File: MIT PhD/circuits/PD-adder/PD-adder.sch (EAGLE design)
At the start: 51 parts, among them U1 INA105KP, U2 OP27EZ, U3 OP27EZ, U4 OP27EZ, U5 INA105KP, U6 OP27EZ, U7 REF01EZ, U8 OP27EZ

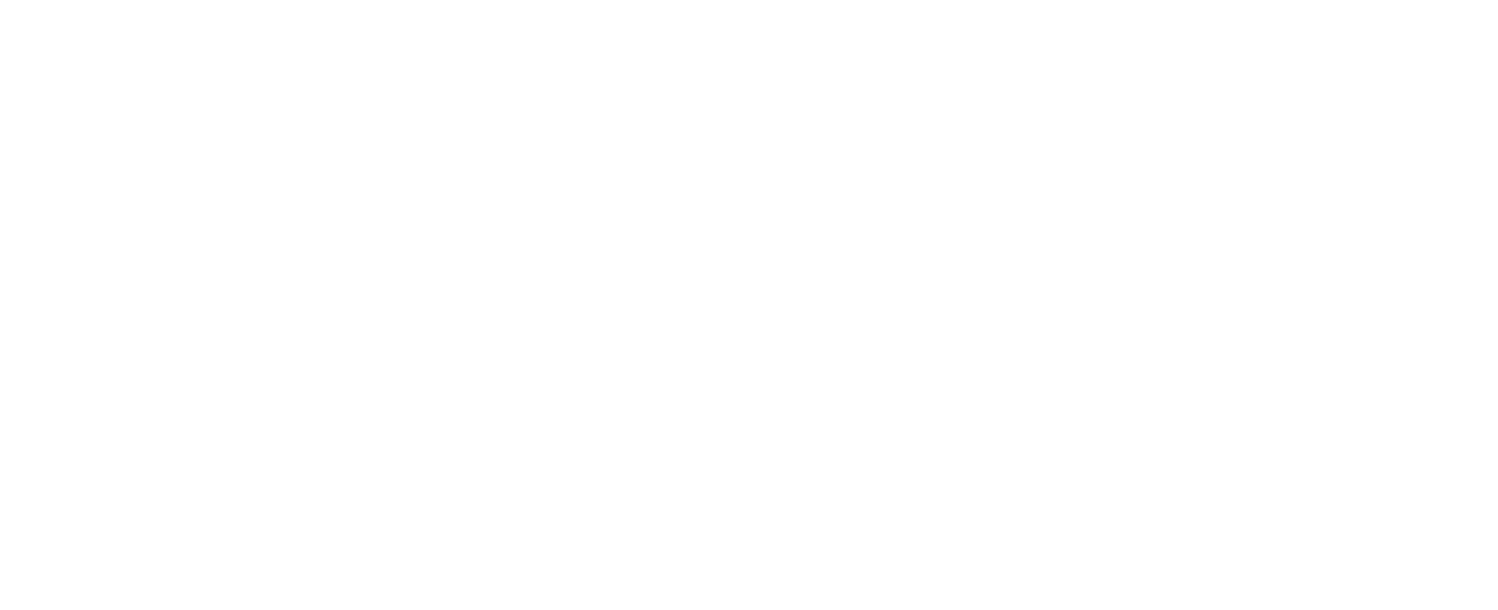
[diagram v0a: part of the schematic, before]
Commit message: circuits
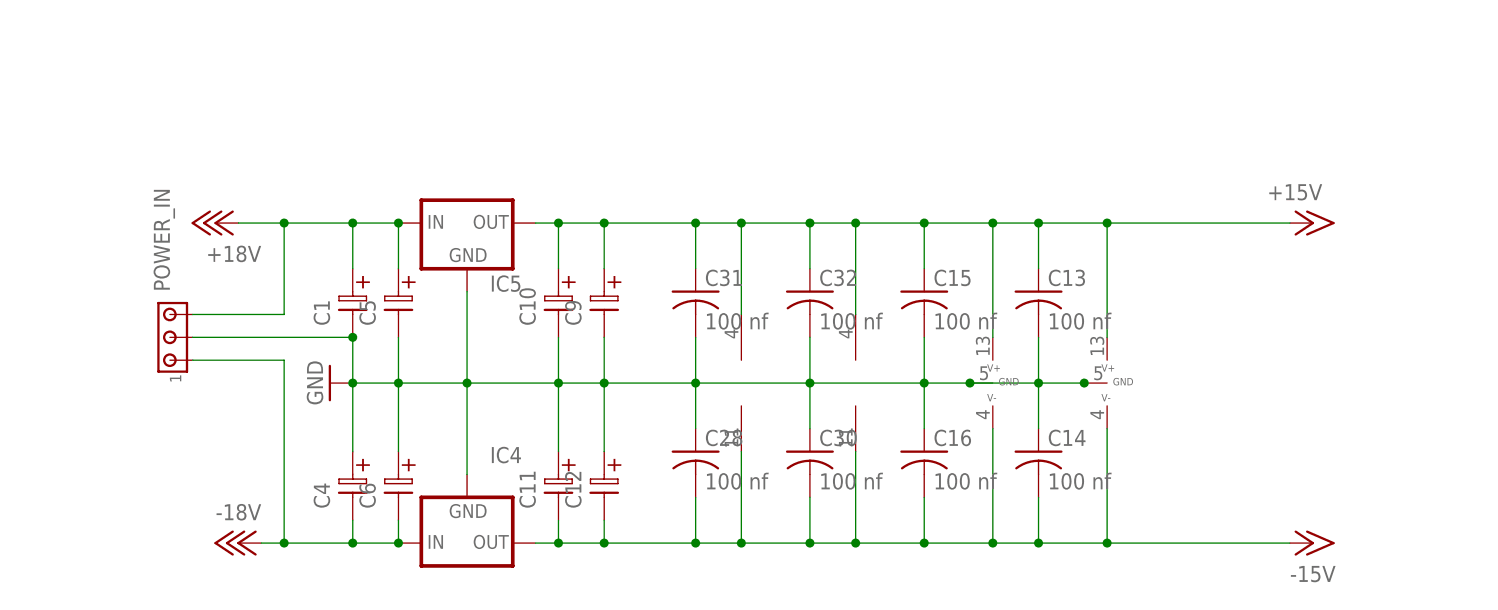
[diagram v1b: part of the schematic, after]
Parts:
- added C1, C10, C11, C12, C4, C5, C6, C9: (no value), discrete:ELC-2,5
- added C13, C14, C15, C16, C28, C30, C31, C32: 100 nf, rcl:C-USC0805
- added IC1: ADG221KN, linear:ADG221KN
- added IC4: (no value), v-reg:79XXL
- added IC5: (no value), v-reg:78XXL
- added IC6, IC7: LF347N, linear:LF347N
- added IC8: ADG222KN, linear:ADG222KN
- added POWER_IN: (no value), con-amp:MTA03-100
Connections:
- new net +18V: C1.1, C5.1, IC5.IN, POWER_IN.3
- new net -18V: C4.2, C6.2, IC4.IN, POWER_IN.1
- net +15V: now also C10.1, C13.1, C15.1, C31.1, C32.1, C9.1, IC1P.V+, IC5.OUT, IC6P.V+, IC7P.V+, IC8P.V+
- net -15V: now also C11.2, C12.2, C14.2, C16.2, C28.2, C30.2, IC1P.V-, IC4.OUT, IC6P.V-, IC7P.V-, IC8P.V-
- net GND: now also C1.2, C10.2, C11.1, C12.1, C13.2, C14.1, C15.2, C16.1, C28.1, C30.1, C31.2, C32.2, C4.1, C5.2, C6.1, C9.2, IC1P.GND, IC4.GND, IC5.GND, IC8P.GND, POWER_IN.2

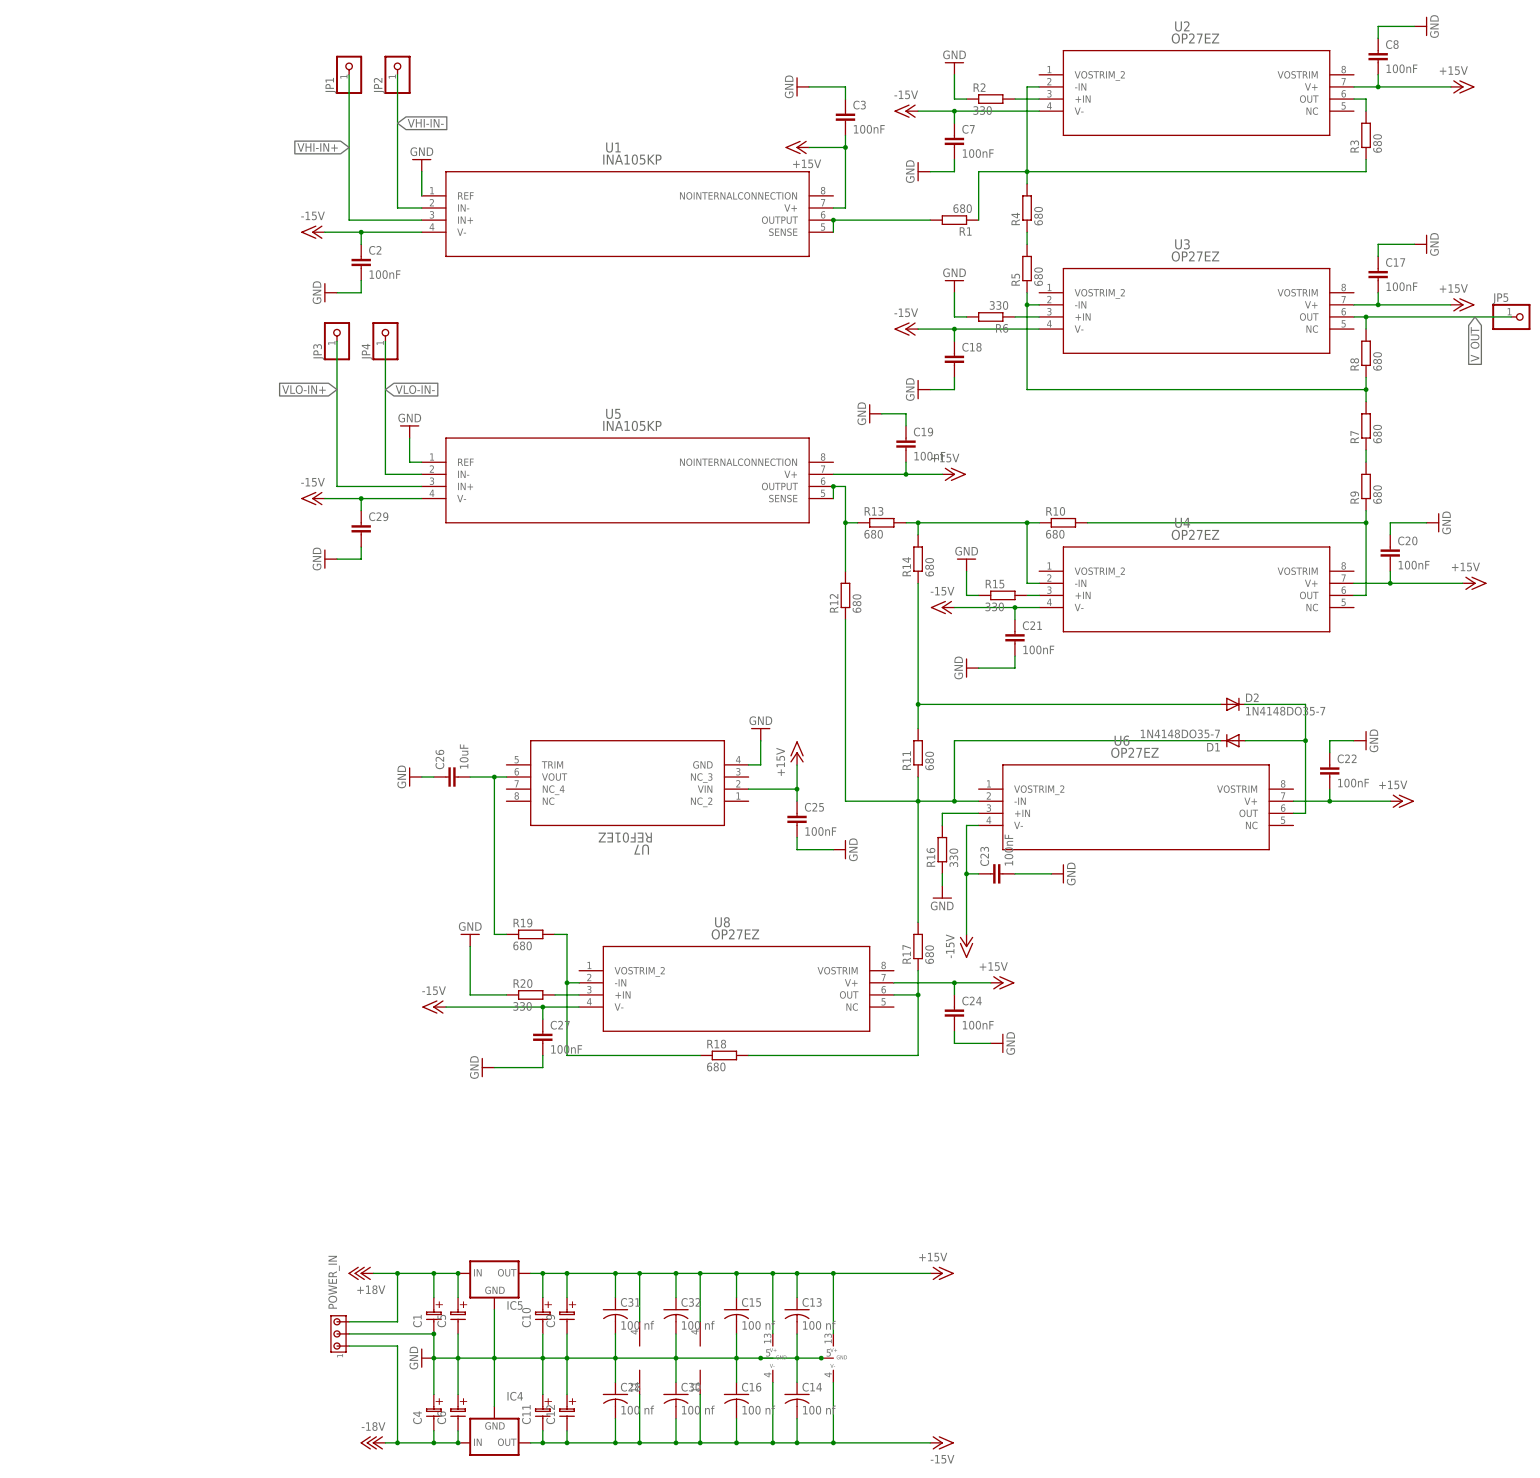
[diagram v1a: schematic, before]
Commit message: circuits
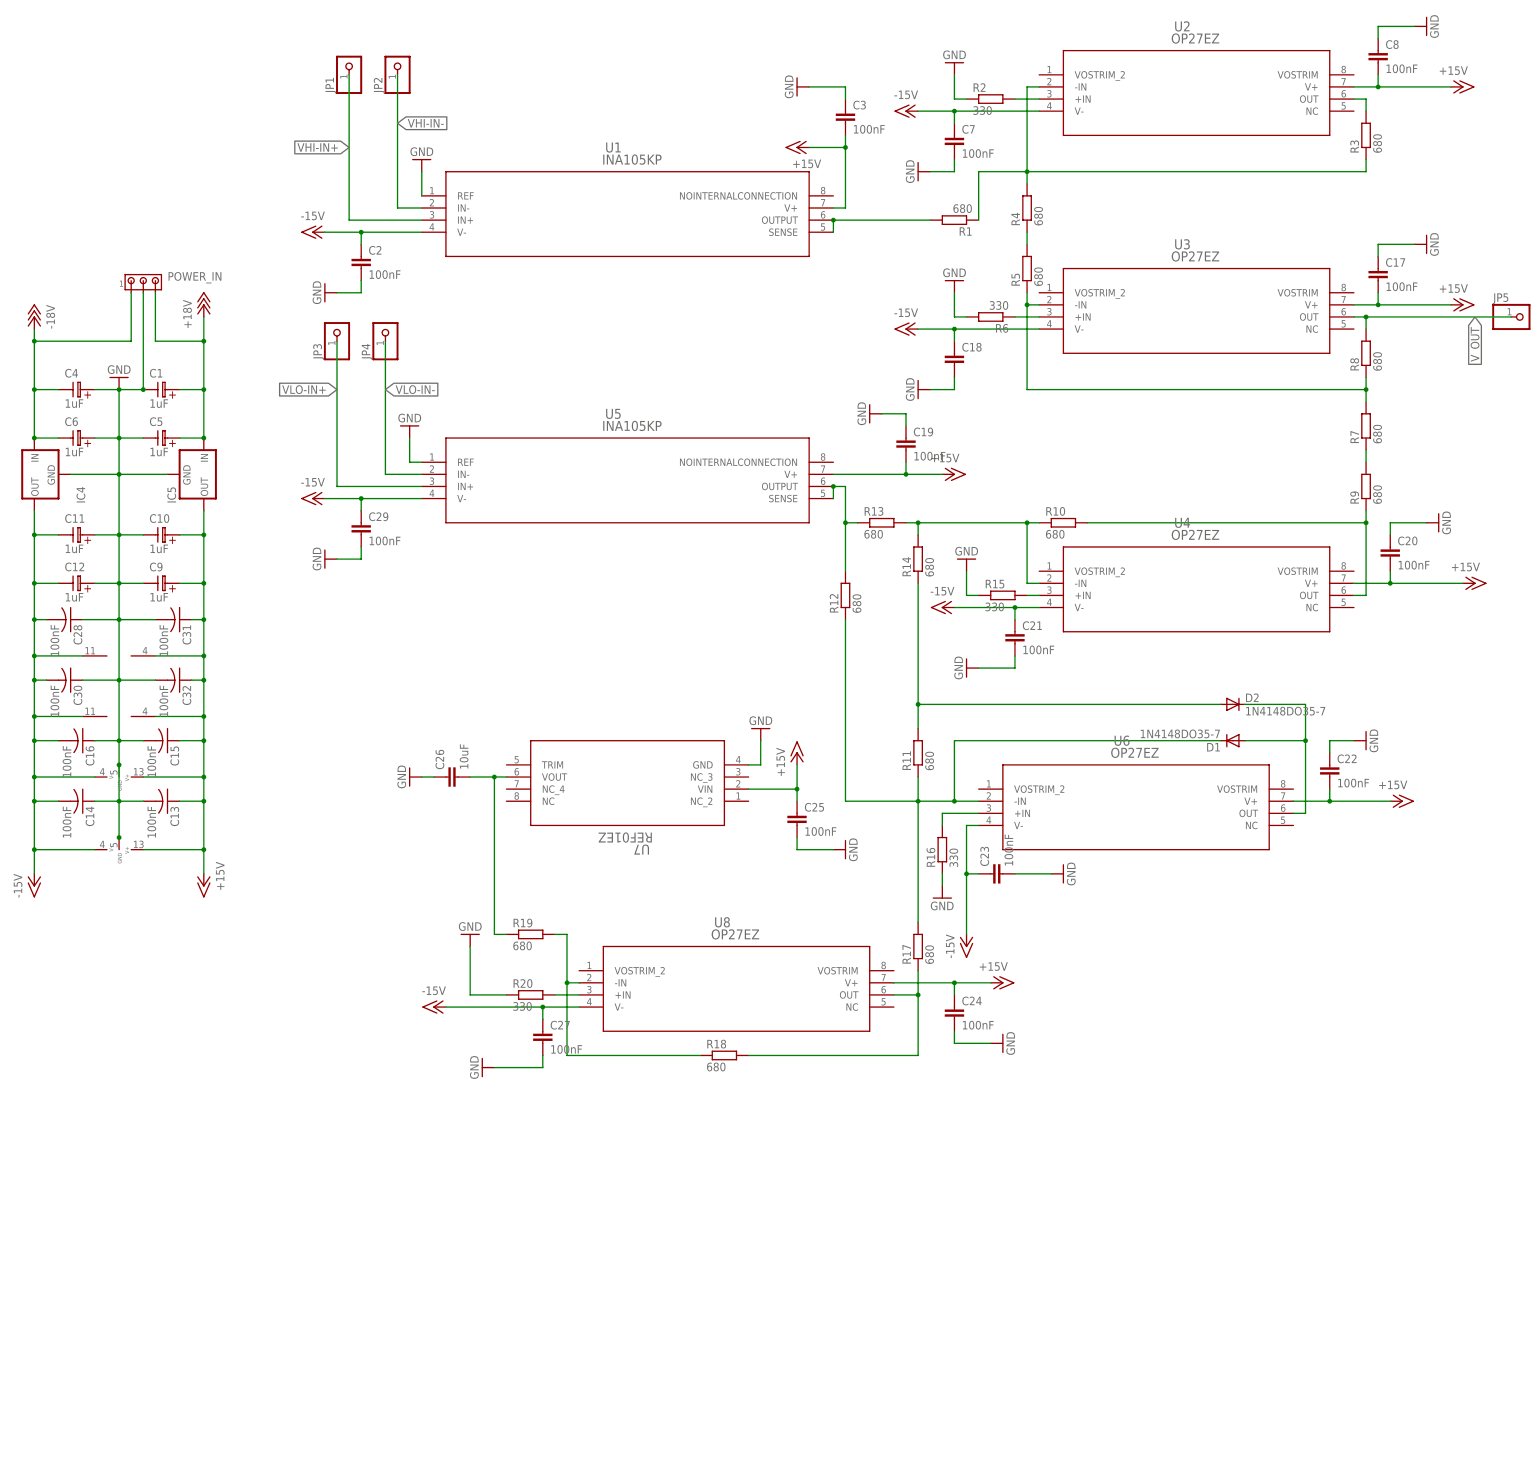
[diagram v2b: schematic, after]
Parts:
- C1, C10, C11, C12, C4, C5, C6, C9: value (none) -> 1uF
- C13, C14, C15, C16, C28, C30, C31, C32: value 100 nf -> 100nF
- C29: value (none) -> 100nF
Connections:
- new net N$1: C13.2, C14.1, IC1P.GND
- net GND: no longer C13.2, C14.1, IC1P.GND
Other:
- moved on the sheet: C1, C10, C11, C12, C13, C14, C15, C16, C28, C30, C31, C32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
